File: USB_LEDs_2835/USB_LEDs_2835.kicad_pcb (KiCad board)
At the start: 2 copper layers, 99.9 x 20 mm, 55 parts, among them U1 MT9284, U2 JL8022W-L, U3 74LVC1G04

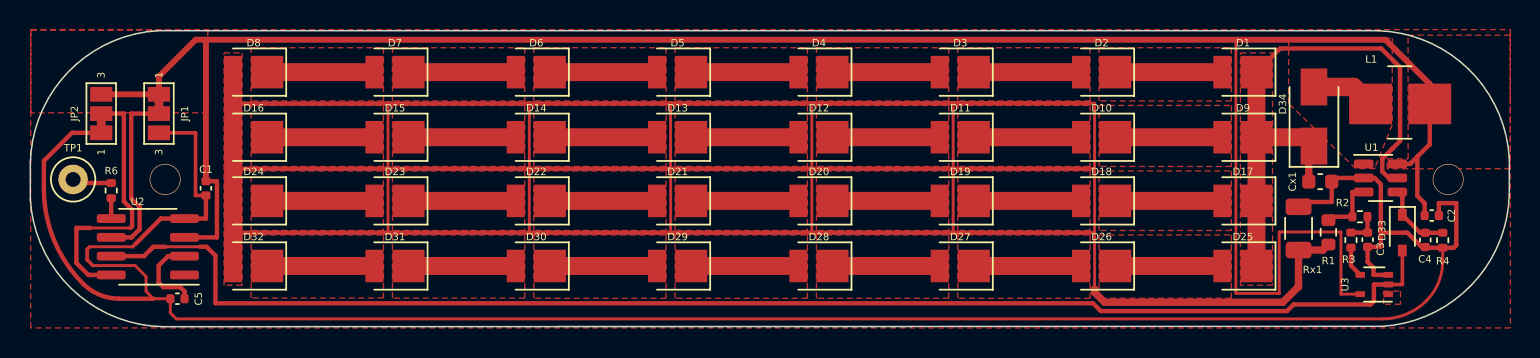
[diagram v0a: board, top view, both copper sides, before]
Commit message: Add files via upload
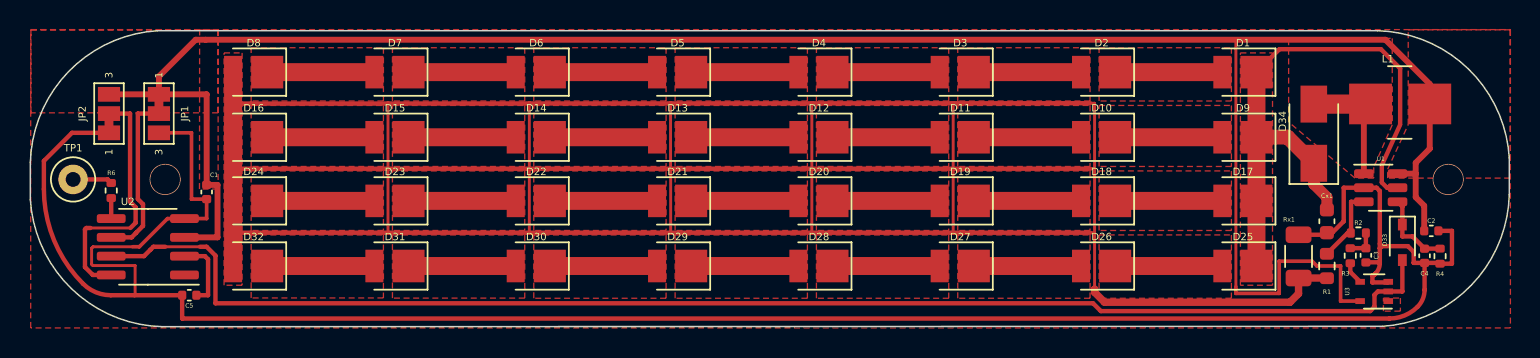
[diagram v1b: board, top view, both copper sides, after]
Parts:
- moved Cx1 2.71 mm to (118.7, 46.5), turned to -90 degrees
- moved R1 2.28 mm to (118.7, 49.5)
- moved Rx1 1.89 mm to (116.8, 48.9)
- moved D34 1.16 mm to (117.8, 40.6)
- moved R2 1.11 mm to (120.8, 47.3)
- moved R4 1.09 mm to (126.3, 48.9)
- moved C4 1.08 mm to (125.3, 48.9)
- moved C3 1.06 mm to (121.3, 48.8)
- moved R3 1.06 mm to (120.3, 48.9)
- moved C2 1.04 mm to (125.7, 47.2)
- moved C5 0.83 mm to (41.8, 51.5)
- moved U1 0.66 mm to (122.3, 44.3)
- moved D33 0.65 mm to (123.8, 47.8)
- moved JP2 0.52 mm to (36.4, 39.2)
- moved U3 0.47 mm to (121.9, 51.3)
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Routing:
- net Net-(D34-Pad2): track 4.30 -> 8.74 mm
- net +5V: track 154.5 -> 150.7 mm
- net GND: track 160.6 -> 158.7 mm
- net Net-(D16-Pad1): track 261.6 -> 259.8 mm
- net Net-(Cx1-Pad1): track 39.4 -> 41.3 mm
- net Net-(JP2-Pad2): track 18.2 -> 17.1 mm
- net Net-(R1-Pad2): track 4.15 -> 5.19 mm
- net Net-(C5-Pad1): track 5.64 -> 4.90 mm
- net Net-(R3-Pad1): track 2.10 -> 1.53 mm
- net Net-(D33-Pad2): track 94.9 -> 94.3 mm
